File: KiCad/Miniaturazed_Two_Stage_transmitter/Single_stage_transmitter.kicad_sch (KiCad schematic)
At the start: 29 parts

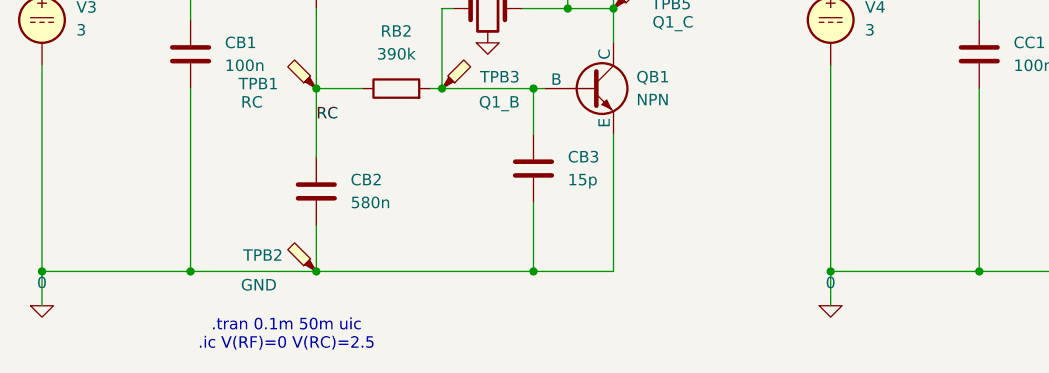
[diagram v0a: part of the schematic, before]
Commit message: pcb cleanup
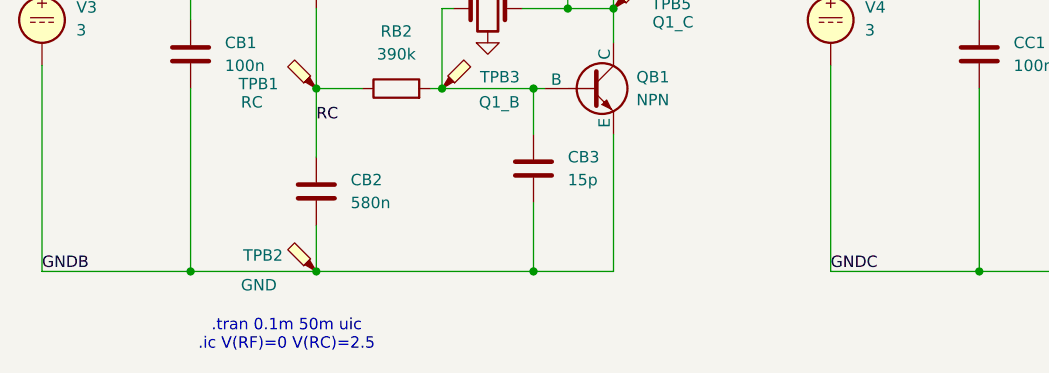
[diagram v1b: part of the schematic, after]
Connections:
- net 0: no longer CB1.2, CB2.2, CB3.2, CC1.2, CC2.2, CC3.2, QB1.3 (E), QC1.3 (E), TPB2.1, V3.2, V4.2
- new net GNDB: CB1.2, CB2.2, CB3.2, QB1.3 (E), TPB2.1, V3.2
- new net GNDC: CC1.2, CC2.2, CC3.2, QC1.3 (E), V4.2
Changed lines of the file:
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@@
-	)
-	(junction
-		(at 74.93 99.06)
-		(diameter 0)
-		(color 0 0 0 0)
-	)
-	(junction
-		(at 162.56 99.06)
-		(diameter 0)
-		(color 0 0 0 0)
 	)
 	(junction
@@
 	(wire
 		(pts
-			(xy 162.56 102.87) (xy 162.56 99.06)
-		)
-		(stroke
-			(width 0)
-			(type default)
-		)
-	)
-	(wire
-		(pts
 			(xy 179.07 71.12) (xy 179.07 40.64)
 		)
@@
 		(pts
 			(xy 129.54 99.06) (xy 105.41 99.06)
-		)
-		(stroke
-			(width 0)
-			(type default)
-		)
-	)
-	(wire
-		(pts
-			(xy 74.93 102.87) (xy 74.93 99.06)
 		)
 		(stroke
@@
 		)
 	)
+	(label "GNDB"
+		(at 74.93 99.06 0)
+		(effects
+			(font
+				(size 1.27 1.27)
+			)
+			(justify left bottom)
+		)
+	)
 	(label "RC"
 		(at 105.41 82.55 0)
@@
 	(label "RF"
 		(at 146.05 54.61 0)
+		(effects
+			(font
+				(size 1.27 1.27)
+			)
+			(justify left bottom)
+		)
+	)
+	(label "GNDC"
+		(at 162.56 99.06 0)
 		(effects
 			(font
@@
 	)
 	(symbol
-		(lib_id "Simulation_SPICE:0")
-		(at 74.93 102.87 0)
-		(unit 1)
-		(body_style 1)
-		(exclude_from_sim no)
-		(in_bom yes)
-		(on_board yes)
-		(in_pos_files yes)
-		(dnp no)
-		(fields_autoplaced yes)
-		(property "Reference" "#GND03"
-			(at 74.93 107.95 0)
-			(hide yes)
-			(show_name no)
-			(do_not_autoplace no)
-			(effects
-				(font
-					(size 1.27 1.27)
-				)
-			)
-		)
-		(property "Value" "0"
-			(at 74.93 100.33 0)
-			(show_name no)
-			(do_not_autoplace no)
-			(effects
-				(font
-					(size 1.27 1.27)
-				)
-			)
-		)
-		(property "Footprint" ""
-			(at 74.93 102.87 0)
-			(hide yes)
-			(show_name no)
-			(do_not_autoplace no)
-			(effects
-				(font
-					(size 1.27 1.27)
-				)
-			)
-		)
-		(property "Datasheet" "https://ngspice.sourceforge.io/docs/ngspice-html-manual/manual.xhtml#subsec_Circuit_elements__device"
-			(at 74.93 113.03 0)
-			(hide yes)
-			(show_name no)
-			(do_not_autoplace no)
-			(effects
-				(font
-					(size 1.27 1.27)
-				)
-			)
-		)
-		(property "Description" "0V reference potential for simulation"
-			(at 74.93 110.49 0)
-			(hide yes)
-			(show_name no)
-			(do_not_autoplace no)
-			(effects
-				(font
-					(size 1.27 1.27)
-				)
-			)
-		)
-		(pin "1"
-		)
-		(instances
-			(project "Miniaturazed_Two_Stage_transmitter"
-				(path "/1ad9bcac-1f06-4b0d-936c-bb8177e25b39/e8ef4360-4377-4627-9337-300800e3fb7d"
-					(reference "#GND03")
-					(unit 1)
-				)
-			)
-		)
-	)
-	(symbol
 		(lib_id "Device:C")
 		(at 193.04 90.17 0)
@@
 					(unit 1)
 				)
-			)
-		)
-	)
-	(symbol
-		(lib_id "Simulation_SPICE:0")
-		(at 162.56 102.87 0)
-		(unit 1)
-		(body_style 1)
-		(exclude_from_sim no)
-		(in_bom yes)
-		(on_board yes)
-		(in_pos_files yes)
-		(dnp no)
-		(fields_autoplaced yes)
-		(property "Reference" "#GND04"
-			(at 162.56 107.95 0)
-			(hide yes)
-			(show_name no)
-			(do_not_autoplace no)
-			(effects
-				(font
-					(size 1.27 1.27)
-				)
-			)
-		)
-		(property "Value" "0"
-			(at 162.56 100.33 0)
-			(show_name no)
-			(do_not_autoplace no)
-			(effects
-				(font
-					(size 1.27 1.27)
-				)
-			)
-		)
-		(property "Footprint" ""
-			(at 162.56 102.87 0)
-			(hide yes)
-			(show_name no)
-			(do_not_autoplace no)
-			(effects
-				(font
-					(size 1.27 1.27)
-				)
-			)
-		)
-		(property "Datasheet" "https://ngspice.sourceforge.io/docs/ngspice-html-manual/manual.xhtml#subsec_Circuit_elements__device"
-			(at 162.56 113.03 0)
-			(hide yes)
-			(show_name no)
-			(do_not_autoplace no)
-			(effects
-				(font
-					(size 1.27 1.27)
-				)
-			)
-		)
-		(property "Description" "0V reference potential for simulation"
-			(at 162.56 110.49 0)
-			(hide yes)
-			(show_name no)
-			(do_not_autoplace no)
-			(effects
-				(font
-					(size 1.27 1.27)
-				)
-			)
-		)
-		(pin "1"
-		)
-		(instances
-			(project "Miniaturazed_Two_Stage_transmitter"
-				(path "/1ad9bcac-1f06-4b0d-936c-bb8177e25b39/e8ef4360-4377-4627-9337-300800e3fb7d"
-					(reference "#GND04")
-					(unit 1)
-				)

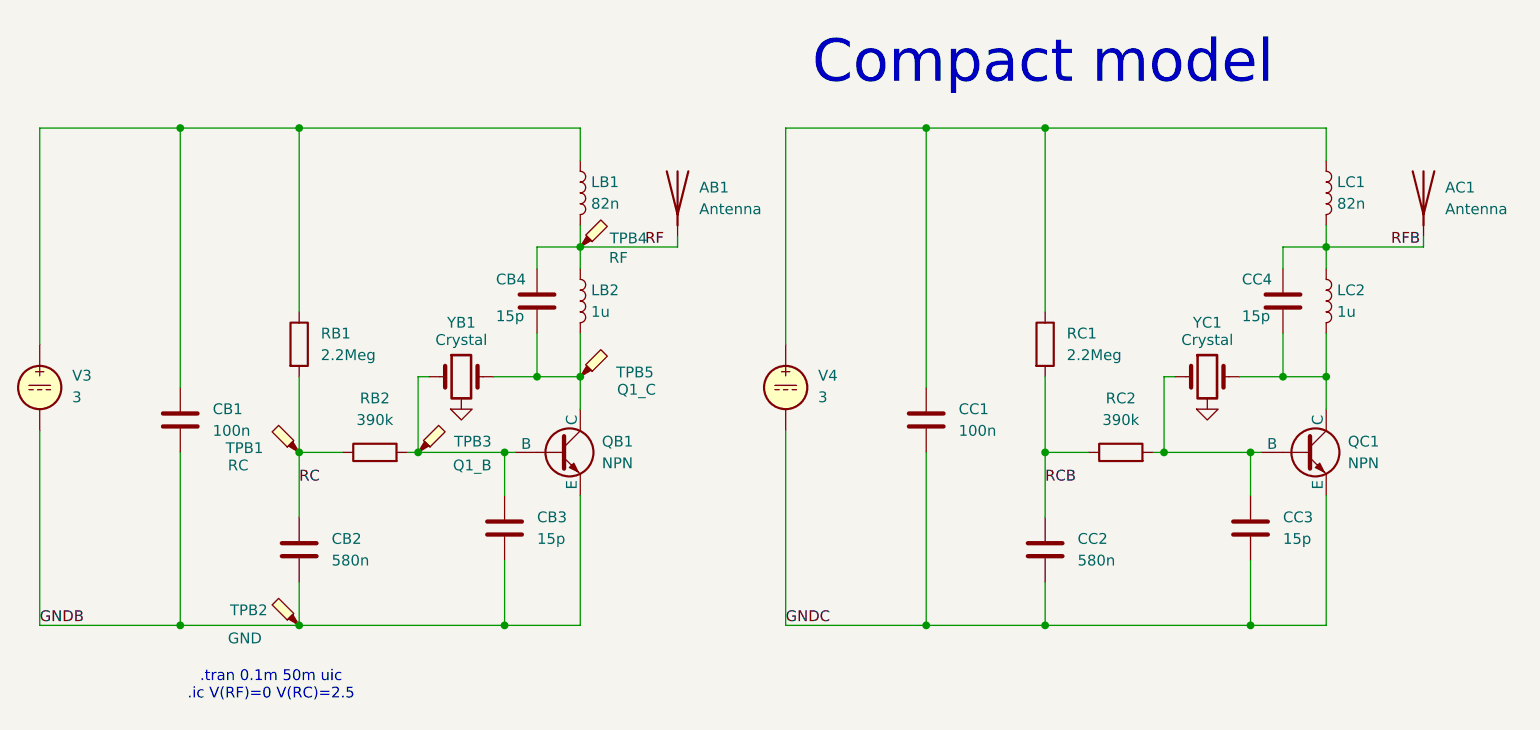
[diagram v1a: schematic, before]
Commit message: modified sst schematic
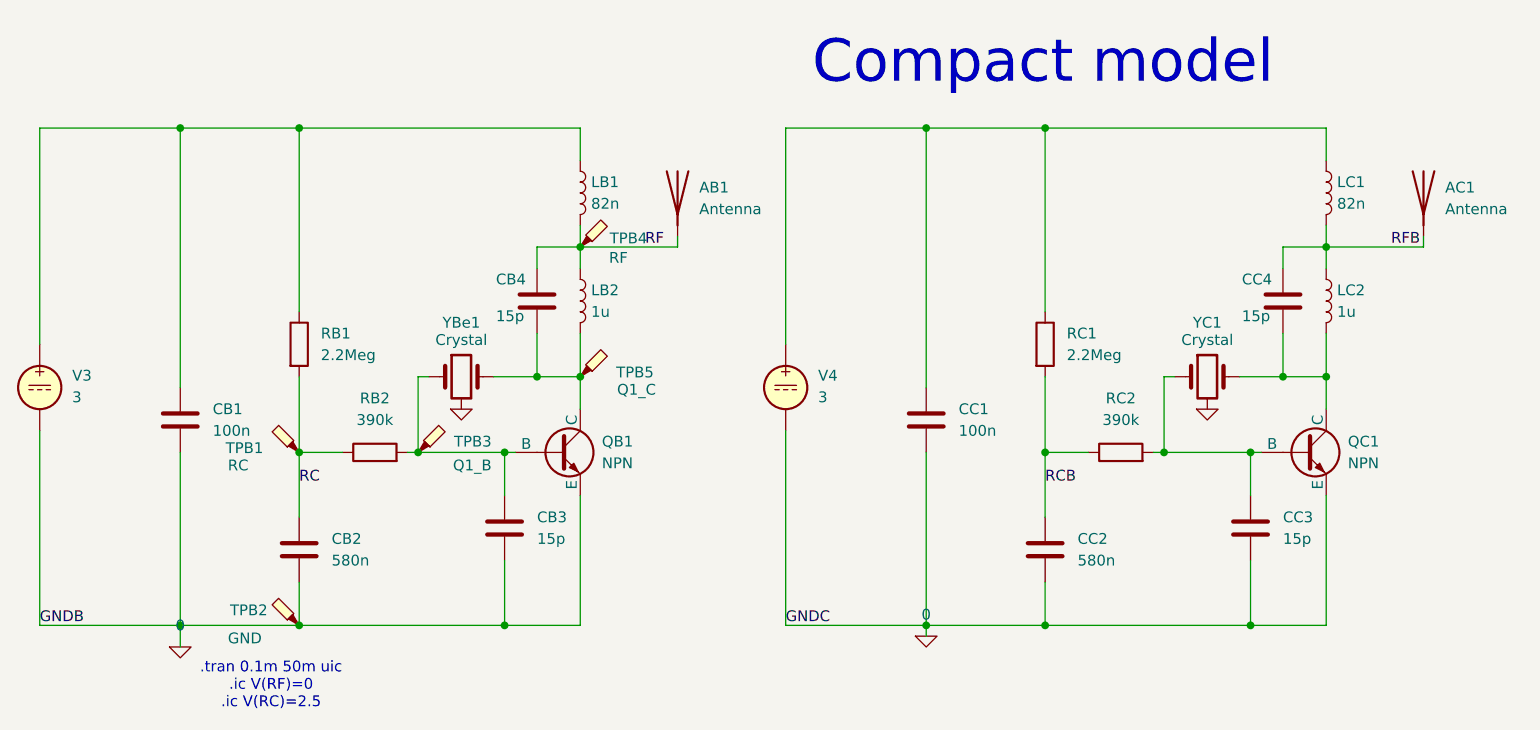
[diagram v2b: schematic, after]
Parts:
- TPB1, TPB2, TPB3, TPB4, TPB5: now left out of the parts list
- renumbered YB1 to YBe1
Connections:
- net GNDB is gone; now on net 0: CB1.2, CB2.2, CB3.2, QB1.3 (E), TPB2.1, V3.2
- net GNDC is gone; now on net 0: CC1.2, CC2.2, CC3.2, QC1.3 (E), V4.2
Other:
- note added: ".tran 0.1m 50m uic .ic V(RF)=0 .ic V(RC)=2.5"
- note removed: ".tran 0.1m 50m uic .ic V(RF)=0 V(RC)=2.5"
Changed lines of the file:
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@@
 	(generator_version "10.0")
 	(paper "A4")
-	(text ".tran 0.1m 50m uic\n.ic V(RF)=0 V(RC)=2.5"
+	(text ".tran 0.1m 50m uic\n.ic V(RF)=0\n.ic V(RC)=2.5"
 		(exclude_from_sim no)
 		(at 102.108 106.172 0)
@@
 	(wire
 		(pts
+			(xy 179.07 100.33) (xy 179.07 99.06)
+		)
+		(stroke
+			(width 0)
+			(type default)
+		)
+	)
+	(wire
+		(pts
 			(xy 220.98 64.77) (xy 220.98 69.85)
 		)
@@
 	(wire
 		(pts
+			(xy 91.44 101.6) (xy 91.44 99.06)
+		)
+		(stroke
+			(width 0)
+			(type default)
+		)
+	)
+	(wire
+		(pts
 			(xy 205.74 78.74) (xy 217.17 78.74)
 		)
@@
 		(unit 1)
 		(body_style 1)
-		(exclude_from_sim no)
-		(in_bom yes)
+		(exclude_from_sim yes)
+		(in_bom no)
 		(on_board yes)
 		(in_pos_files yes)
@@
 	)
 	(symbol
+		(lib_id "Simulation_SPICE:0")
+		(at 179.07 100.33 0)
+		(unit 1)
+		(body_style 1)
+		(exclude_from_sim no)
+		(in_bom yes)
+		(on_board yes)
+		(in_pos_files yes)
+		(dnp no)
+		(fields_autoplaced yes)
+		(property "Reference" "#GND05"
+			(at 179.07 105.41 0)
+			(hide yes)
+			(show_name no)
+			(do_not_autoplace no)
+			(effects
+				(font
+					(size 1.27 1.27)
+				)
+			)
+		)
+		(property "Value" "0"
+			(at 179.07 97.79 0)
+			(show_name no)
+			(do_not_autoplace no)
+			(effects
+				(font
+					(size 1.27 1.27)
+				)
+			)
+		)
+		(property "Footprint" ""
+			(at 179.07 100.33 0)
+			(hide yes)
+			(show_name no)
+			(do_not_autoplace no)
+			(effects
+				(font
+					(size 1.27 1.27)
+				)
+			)
+		)
+		(property "Datasheet" "https://ngspice.sourceforge.io/docs/ngspice-html-manual/manual.xhtml#subsec_Circuit_elements__device"
+			(at 179.07 110.49 0)
+			(hide yes)
+			(show_name no)
+			(do_not_autoplace no)
+			(effects
+				(font
+					(size 1.27 1.27)
+				)
+			)
+		)
+		(property "Description" "0V reference potential for simulation"
+			(at 179.07 107.95 0)
+			(hide yes)
+			(show_name no)
+			(do_not_autoplace no)
+			(effects
+				(font
+					(size 1.27 1.27)
+				)
+			)
+		)
+		(pin "1"
+		)
+		(instances
+			(project "Miniaturazed_Two_Stage_transmitter"
+				(path "/1ad9bcac-1f06-4b0d-936c-bb8177e25b39/e8ef4360-4377-4627-9337-300800e3fb7d"
+					(reference "#GND05")
+					(unit 1)
+				)
+			)
+		)
+	)
+	(symbol
 		(lib_id "Device:C")
 		(at 179.07 74.93 0)
 		(unit 1)
 		(body_style 1)
-		(exclude_from_sim no)
+		(exclude_from_sim yes)
 		(in_bom yes)
 		(on_board yes)
@@
 		(unit 1)
 		(body_style 1)
-		(exclude_from_sim no)
+		(exclude_from_sim yes)
 		(in_bom yes)
 		(on_board yes)
@@
 		(unit 1)
 		(body_style 1)
-		(exclude_from_sim no)
-		(in_bom yes)
+		(exclude_from_sim yes)
+		(in_bom no)
 		(on_board yes)
 		(in_pos_files yes)
@@
 		(unit 1)
 		(body_style 1)
-		(exclude_from_sim no)
-		(in_bom yes)
+		(exclude_from_sim yes)
+		(in_bom no)
 		(on_board yes)
 		(in_pos_files yes)
@@
 		(unit 1)
 		(body_style 1)
-		(exclude_from_sim no)
+		(exclude_from_sim yes)
 		(in_bom yes)
 		(on_board yes)
@@
 	)
 	(symbol
+		(lib_id "Simulation_SPICE:0")
+		(at 91.44 101.6 0)
+		(unit 1)
+		(body_style 1)
+		(exclude_from_sim no)
+		(in_bom yes)
+		(on_board yes)
+		(in_pos_files yes)
+		(dnp no)
+		(fields_autoplaced yes)
+		(property "Reference" "#GND03"
+			(at 91.44 106.68 0)
+			(hide yes)
+			(show_name no)
+			(do_not_autoplace no)
+			(effects
+				(font
+					(size 1.27 1.27)
+				)
+			)
+		)
+		(property "Value" "0"
+			(at 91.44 99.06 0)
+			(show_name no)
+			(do_not_autoplace no)
+			(effects
+				(font
+					(size 1.27 1.27)
+				)
+			)
+		)
+		(property "Footprint" ""
+			(at 91.44 101.6 0)
+			(hide yes)
+			(show_name no)
+			(do_not_autoplace no)
+			(effects
+				(font
+					(size 1.27 1.27)
+				)
+			)
+		)
+		(property "Datasheet" "https://ngspice.sourceforge.io/docs/ngspice-html-manual/manual.xhtml#subsec_Circuit_elements__device"
+			(at 91.44 111.76 0)
+			(hide yes)
+			(show_name no)
+			(do_not_autoplace no)
+			(effects
+				(font
+					(size 1.27 1.27)
+				)
+			)
+		)
+		(property "Description" "0V reference potential for simulation"
+			(at 91.44 109.22 0)
+			(hide yes)
+			(show_name no)
+			(do_not_autoplace no)
+			(effects
+				(font
+					(size 1.27 1.27)
+				)
+			)
+		)
+		(pin "1"
+		)
+		(instances
+			(project "Miniaturazed_Two_Stage_transmitter"
+				(path "/1ad9bcac-1f06-4b0d-936c-bb8177e25b39/e8ef4360-4377-4627-9337-300800e3fb7d"
+					(reference "#GND03")
+					(unit 1)
+				)
+			)
+		)
+	)
+	(symbol
 		(lib_id "Device:L")
 		(at 138.43 48.26 0)
@@
 		(unit 1)
 		(body_style 1)
-		(exclude_from_sim no)
+		(exclude_from_sim yes)
 		(in_bom yes)
 		(on_board yes)
@@
 			)
 		)
-		(property "Sim.Pins" "1=1 2=2"
+		(property "Sim.Pins" "2=2 4=1"
 			(at 212.09 69.85 0)
 			(hide yes)
@@
 		(unit 1)
 		(body_style 1)
-		(exclude_from_sim no)
+		(exclude_from_sim yes)
 		(in_bom yes)
 		(on_board yes)
@@
 		(unit 1)
 		(body_style 1)
-		(exclude_from_sim no)
+		(exclude_from_sim yes)
 		(in_bom yes)
 		(on_board yes)
@@
 		(in_pos_files yes)
 		(dnp no)
-		(property "Reference" "YB1"
+		(property "Reference" "YBe1"
 			(at 124.46 63.5 0)
 			(show_name no)
@@
 			)
 		)
-		(property "Sim.Pins" "1=1 2=2"
+		(property "Sim.Pins" "2=2 3=3 4=1"
 			(at 124.46 69.85 0)
 			(hide yes)
@@
 			(project "Miniaturazed_Two_Stage_transmitter"
 				(path "/1ad9bcac-1f06-4b0d-936c-bb8177e25b39/e8ef4360-4377-4627-9337-300800e3fb7d"
-					(reference "YB1")
+					(reference "YBe1")
 					(unit 1)
 				)
@@
 		(unit 1)
 		(body_style 1)
-		(exclude_from_sim no)
+		(exclude_from_sim yes)
 		(in_bom yes)
 		(on_board yes)
@@
 		(unit 1)
 		(body_style 1)
-		(exclude_from_sim no)
+		(exclude_from_sim yes)
 		(in_bom yes)
 		(on_board yes)
@@
 		(unit 1)
 		(body_style 1)
-		(exclude_from_sim no)
-		(in_bom yes)
+		(exclude_from_sim yes)
+		(in_bom no)
 		(on_board yes)
 		(in_pos_files yes)
@@
 		(unit 1)
 		(body_style 1)
-		(exclude_from_sim no)
+		(exclude_from_sim yes)
 		(in_bom yes)
 		(on_board yes)
@@
 		(dnp no)
 		(fields_autoplaced yes)
-		(property "Reference" "#GND06"
+		(property "Reference" "#GND04"
 			(at 124.46 78.74 0)
 			(hide yes)
@@
 			(project "Miniaturazed_Two_Stage_transmitter"
 				(path "/1ad9bcac-1f06-4b0d-936c-bb8177e25b39/e8ef4360-4377-4627-9337-300800e3fb7d"
-					(reference "#GND06")
+					(reference "#GND04")
 					(unit 1)
 				)
@@
 		(unit 1)
 		(body_style 1)
-		(exclude_from_sim no)
+		(exclude_from_sim yes)
 		(in_bom yes)
 		(on_board yes)
@@
 		(unit 1)
 		(body_style 1)
-		(exclude_from_sim no)
-		(in_bom yes)
+		(exclude_from_sim yes)
+		(in_bom no)
 		(on_board yes)
 		(in_pos_files yes)
@@
 		(unit 1)
 		(body_style 1)
-		(exclude_from_sim no)
+		(exclude_from_sim yes)
 		(in_bom yes)
 		(on_board yes)
@@
 		(dnp no)
 		(fields_autoplaced yes)
-		(property "Reference" "#GND07"
+		(property "Reference" "#GND06"
 			(at 212.09 78.74 0)
 			(hide yes)
@@
 			(project "Miniaturazed_Two_Stage_transmitter"
 				(path "/1ad9bcac-1f06-4b0d-936c-bb8177e25b39/e8ef4360-4377-4627-9337-300800e3fb7d"
-					(reference "#GND07")
+					(reference "#GND06")
 					(unit 1)
 				)
@@
 		(unit 1)
 		(body_style 1)
-		(exclude_from_sim no)
+		(exclude_from_sim yes)
 		(in_bom yes)
 		(on_board yes)
